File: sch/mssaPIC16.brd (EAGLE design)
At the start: 60.2 x 30 mm, 32 parts, among them IC1 PIC16F676P, IC2 7805L, Q1 BC550C, Q2 BC550C

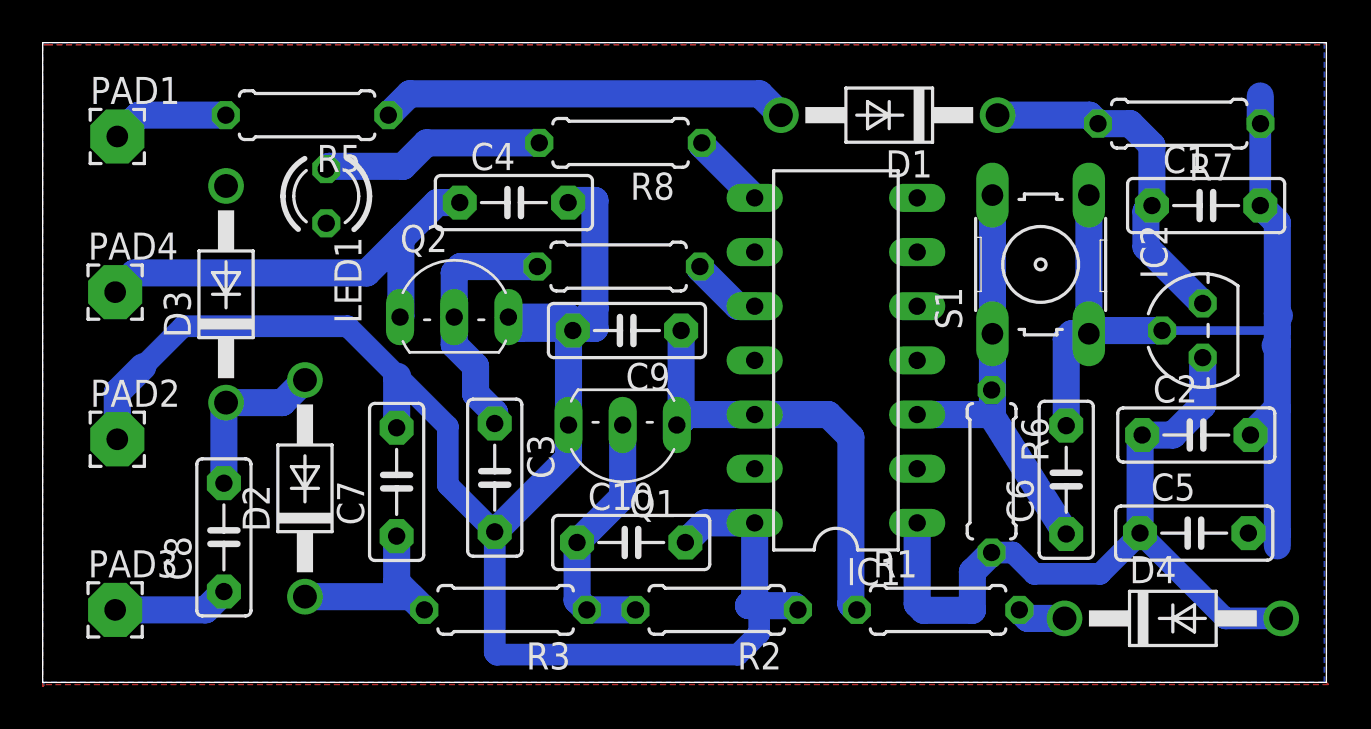
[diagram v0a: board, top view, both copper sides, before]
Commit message: SSA v.034
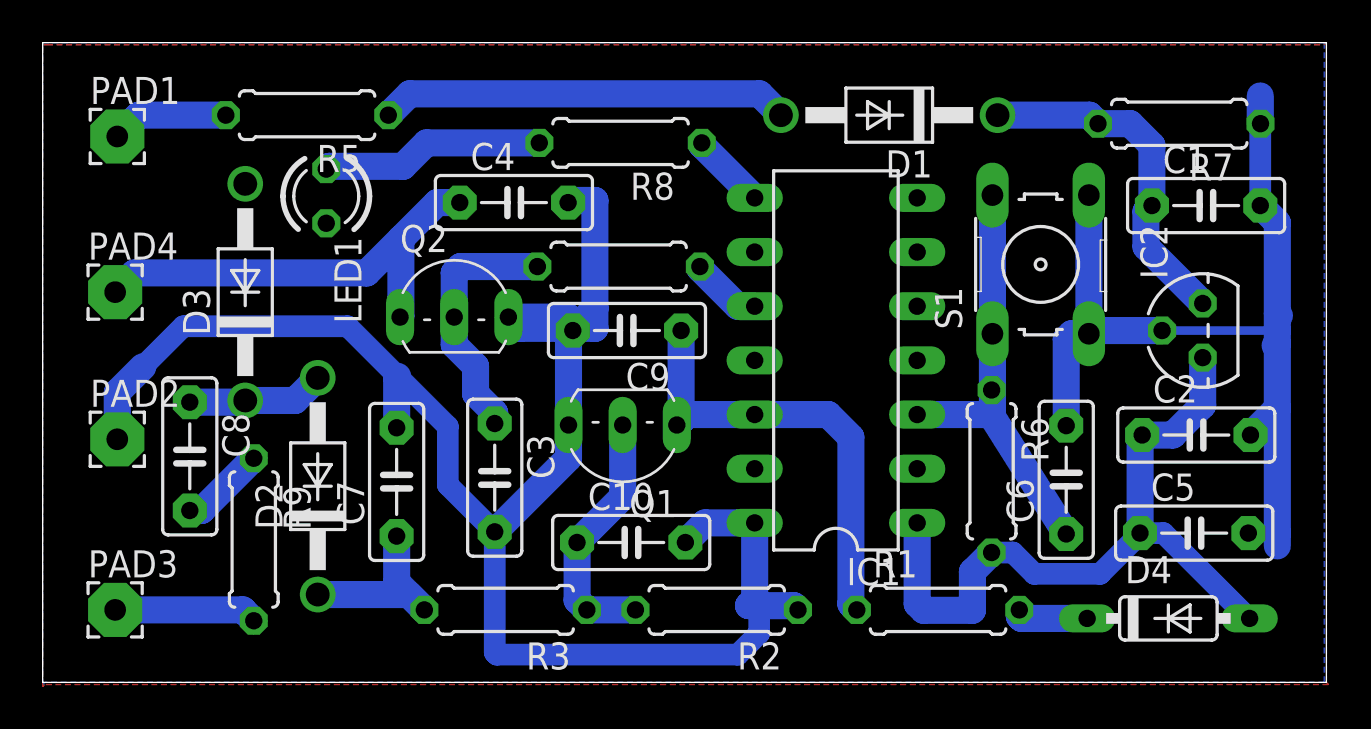
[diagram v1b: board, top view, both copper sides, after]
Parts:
- added R9: 100, rcl:0207/7
- D4: value 1N4004 -> 1N4148DO35-7; device diode:DO41-10 -> diode:DO35-7
- moved C8 4.12 mm to (6.90, 10.6), turned to 270 degrees
- moved D3 0.91 mm to (9.50, 18.3)
- moved D2 0.61 mm to (12.9, 9.20)
- moved D4 0.21 mm to (52.8, 3.00)
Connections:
- new net N$17: PAD3.1, R9.2
- net N$12: now also C8.2, R9.1; no longer C8.1, PAD3.1
- net N$13: now also C8.1; no longer C8.2
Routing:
- net N$17: track 0.00 -> 6.71 mm
- net N$2: track 36.4 -> 34.9 mm
- net N$13: track 7.96 -> 6.49 mm
- net N$12: track 5.46 -> 4.01 mm
- net N$16: track 2.29 -> 3.52 mm
- net N$9: track 9.86 -> 9.30 mm
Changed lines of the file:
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@@
 <setting verticaltext="up"/>
 </settings>
-<grid distance="1" unitdist="mm" unit="mm" style="lines" multiple="10" display="yes" altdistance="1" altunitdist="mm" altunit="mm"/>
+<grid distance="0.1" unitdist="mm" unit="mm" style="lines" multiple="10" display="yes" altdistance="1" altunitdist="mm" altunit="mm"/>
 <layers>
 <layer number="1" name="Top" color="11" fill="1" visible="yes" active="yes"/>
@@
 <attribute name="VALUE" x="19.394" y="7.368" size="1.27" layer="27" ratio="10" rot="R90"/>
 </element>
-<element name="D2" library="diode" library_urn="urn:adsk.eagle:library:210" package="DO41-10" package3d_urn="urn:adsk.eagle:package:43336/1" value="1N4004" x="12.3" y="9.1" smashed="yes" rot="R90">
-<attribute name="NAME" x="10.649" y="7.068" size="1.27" layer="25" ratio="10" rot="R90"/>
-<attribute name="POPULARITY" value="82" x="12.3" y="9.1" size="1.778" layer="27" rot="R90" display="off"/>
-<attribute name="VALUE" x="15.094" y="7.068" size="1.27" layer="27" ratio="10" rot="R90"/>
-</element>
-<element name="D3" library="diode" library_urn="urn:adsk.eagle:library:210" package="DO41-10" package3d_urn="urn:adsk.eagle:package:43336/1" value="1N4004" x="8.6" y="18.2" smashed="yes" rot="R90">
-<attribute name="NAME" x="6.949" y="16.168" size="1.27" layer="25" ratio="10" rot="R90"/>
-<attribute name="POPULARITY" value="82" x="8.6" y="18.2" size="1.778" layer="27" rot="R90" display="off"/>
-<attribute name="VALUE" x="11.394" y="16.168" size="1.27" layer="27" ratio="10" rot="R90"/>
-</element>
-<element name="C8" library="capacitor-wima" package="C5B2.5" value="220n" x="8.5" y="6.8" smashed="yes" rot="R90">
-<attribute name="NAME" x="6.976" y="4.768" size="1.27" layer="25" ratio="10" rot="R90"/>
-<attribute name="VALUE" x="11.294" y="4.768" size="1.27" layer="27" ratio="10" rot="R90"/>
+<element name="D2" library="diode" library_urn="urn:adsk.eagle:library:210" package="DO41-10" package3d_urn="urn:adsk.eagle:package:43336/1" value="1N4004" x="12.9" y="9.2" smashed="yes" rot="R90">
+<attribute name="NAME" x="11.249" y="7.168" size="1.27" layer="25" ratio="10" rot="R90"/>
+<attribute name="POPULARITY" value="82" x="12.9" y="9.2" size="1.778" layer="27" rot="R90" display="off"/>
+<attribute name="VALUE" x="15.694" y="7.168" size="1.27" layer="27" ratio="10" rot="R90"/>
+</element>
+<element name="D3" library="diode" library_urn="urn:adsk.eagle:library:210" package="DO41-10" package3d_urn="urn:adsk.eagle:package:43336/1" value="1N4004" x="9.5" y="18.3" smashed="yes" rot="R90">
+<attribute name="NAME" x="7.849" y="16.268" size="1.27" layer="25" ratio="10" rot="R90"/>
+<attribute name="POPULARITY" value="82" x="9.5" y="18.3" size="1.778" layer="27" rot="R90" display="off"/>
+<attribute name="VALUE" x="12.294" y="16.268" size="1.27" layer="27" ratio="10" rot="R90"/>
+</element>
+<element name="C8" library="capacitor-wima" package="C5B2.5" value="220n" x="6.9" y="10.6" smashed="yes" rot="R270">
+<attribute name="NAME" x="8.424" y="12.632" size="1.27" layer="25" ratio="10" rot="R270"/>
+<attribute name="VALUE" x="4.106" y="12.632" size="1.27" layer="27" ratio="10" rot="R270"/>
 </element>
 <element name="C9" library="capacitor-wima" package="C5B2.5" value="2.2u" x="27.4" y="16.5" smashed="yes" rot="R180">
@@
 <attribute name="VALUE" x="11.649" y="20.895" size="1.27" layer="27" ratio="10" rot="R270"/>
 </element>
-<element name="D4" library="diode" library_urn="urn:adsk.eagle:library:210" package="DO41-10" package3d_urn="urn:adsk.eagle:package:43336/1" value="1N4004" x="53" y="3" smashed="yes">
-<attribute name="NAME" x="50.968" y="4.651" size="1.27" layer="25" ratio="10"/>
-<attribute name="POPULARITY" value="82" x="53" y="3" size="1.778" layer="27" display="off"/>
-<attribute name="VALUE" x="50.968" y="0.206" size="1.27" layer="27" ratio="10"/>
+<element name="D4" library="diode" library_urn="urn:adsk.eagle:library:210" package="DO35-7" package3d_urn="urn:adsk.eagle:package:43339/2" value="1N4148DO35-7" x="52.79" y="3" smashed="yes">
+<attribute name="NAME" x="50.758" y="4.651" size="1.27" layer="25" ratio="10"/>
+<attribute name="POPULARITY" value="58" x="52.79" y="3" size="1.778" layer="27" display="off"/>
+<attribute name="VALUE" x="50.758" y="0.206" size="1.27" layer="27" ratio="10"/>
+</element>
+<element name="R9" library="rcl" library_urn="urn:adsk.eagle:library:334" package="0207/7" package3d_urn="urn:adsk.eagle:package:23493/2" value="100" x="9.9" y="6.7" smashed="yes" rot="R270">
+<attribute name="NAME" x="11.297" y="9.24" size="1.27" layer="25" ratio="10" rot="R270"/>
+<attribute name="POPULARITY" value="46" x="9.9" y="6.7" size="1.778" layer="27" rot="R270" display="off"/>
+<attribute name="SPICEPREFIX" value="R" x="9.9" y="6.7" size="1.778" layer="27" rot="R270" display="off"/>
+<attribute name="VALUE" x="9.3412" y="8.986" size="1.27" layer="27" ratio="10" rot="R270"/>
 </element>
 </elements>
@@
 <wire x1="44.5" y1="6.09" x2="45.5" y2="6.09" width="1.016" layer="16"/>
 <wire x1="49.59" y1="5.09" x2="51.46" y2="6.96" width="1.016" layer="16"/>
-<wire x1="58.08" y1="3" x2="55.46" y2="3" width="1.016" layer="16"/>
-<wire x1="55.46" y1="3" x2="51.46" y2="7" width="1.016" layer="16"/>
+<wire x1="56.6" y1="3" x2="56.56" y2="3" width="1.016" layer="16"/>
+<wire x1="56.56" y1="3" x2="52.56" y2="7" width="1.016" layer="16"/>
+<wire x1="52.56" y1="7" x2="51.46" y2="7" width="1.016" layer="16"/>
 </signal>
 <signal name="N$3">
@@
 <contactref element="C7" pad="1"/>
 <contactref element="D2" pad="C"/>
-<wire x1="12.3" y1="4.02" x2="17.28" y2="4.02" width="1.27" layer="16"/>
-<wire x1="17.28" y1="4.02" x2="17.9" y2="3.4" width="1.27" layer="16"/>
+<wire x1="12.9" y1="4.12" x2="17.18" y2="4.12" width="1.27" layer="16"/>
+<wire x1="17.18" y1="4.12" x2="17.9" y2="3.4" width="1.27" layer="16"/>
 <wire x1="17.9" y1="3.4" x2="16.6" y2="4.7" width="1.27" layer="16"/>
 <wire x1="16.6" y1="4.7" x2="16.6" y2="6.86" width="1.27" layer="16"/>
@@
 <contactref element="D3" pad="C"/>
 <contactref element="D2" pad="A"/>
-<contactref element="C8" pad="2"/>
-<wire x1="8.5" y1="9.34" x2="8.5" y2="13.02" width="1.27" layer="16"/>
-<wire x1="8.5" y1="13.02" x2="8.6" y2="13.12" width="1.27" layer="16"/>
-<wire x1="8.6" y1="13.12" x2="11.24" y2="13.12" width="1.27" layer="16"/>
-<wire x1="11.24" y1="13.12" x2="12.3" y2="14.18" width="1.27" layer="16"/>
-</signal>
-<signal name="N$12">
+<wire x1="9.4" y1="13.12" x2="9.5" y2="13.22" width="1.27" layer="16"/>
+<wire x1="9.5" y1="13.22" x2="11.84" y2="13.22" width="1.27" layer="16"/>
+<wire x1="11.84" y1="13.22" x2="12.9" y2="14.28" width="1.27" layer="16"/>
 <contactref element="C8" pad="1"/>
-<contactref element="PAD3" pad="1"/>
-<wire x1="3.4" y1="3.4" x2="7.64" y2="3.4" width="1.27" layer="16"/>
-<wire x1="7.64" y1="3.4" x2="8.5" y2="4.26" width="1.27" layer="16"/>
+<wire x1="6.9" y1="13.14" x2="9.38" y2="13.14" width="1.27" layer="16"/>
+<wire x1="9.38" y1="13.14" x2="9.4" y2="13.12" width="1.27" layer="16"/>
 </signal>
 <signal name="N$14">
@@
 <contactref element="R1" pad="2"/>
 <contactref element="D4" pad="C"/>
-<wire x1="45.8" y1="3.4" x2="46.2" y2="3" width="1.27" layer="16"/>
-<wire x1="46.2" y1="3" x2="47.92" y2="3" width="1.27" layer="16"/>
+<wire x1="45.8" y1="3.4" x2="45.8" y2="3.1" width="1.27" layer="16"/>
+<wire x1="45.9" y1="3" x2="45.8" y2="3.1" width="1.27" layer="16"/>
+<wire x1="45.9" y1="3" x2="48.98" y2="3" width="1.27" layer="16"/>
+</signal>
+<signal name="N$12">
+<contactref element="R9" pad="1"/>
+<contactref element="C8" pad="2"/>
+<wire x1="6.9" y1="8.06" x2="7.45" y2="8.06" width="1.27" layer="16"/>
+<wire x1="7.45" y1="8.06" x2="9.9" y2="10.51" width="1.27" layer="16"/>
+</signal>
+<signal name="N$17">
+<contactref element="R9" pad="2"/>
+<contactref element="PAD3" pad="1"/>
+<wire x1="3.4" y1="3.4" x2="9.39" y2="3.4" width="1.27" layer="16"/>
+<wire x1="9.39" y1="3.4" x2="9.9" y2="2.89" width="1.27" layer="16"/>
 </signal>
 </signals>

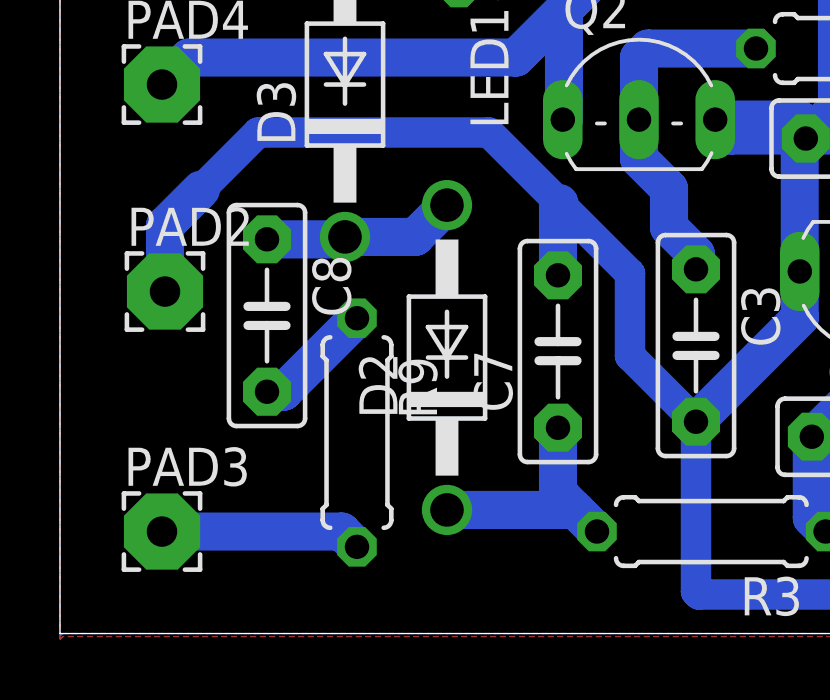
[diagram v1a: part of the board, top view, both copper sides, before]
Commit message: Add files via upload
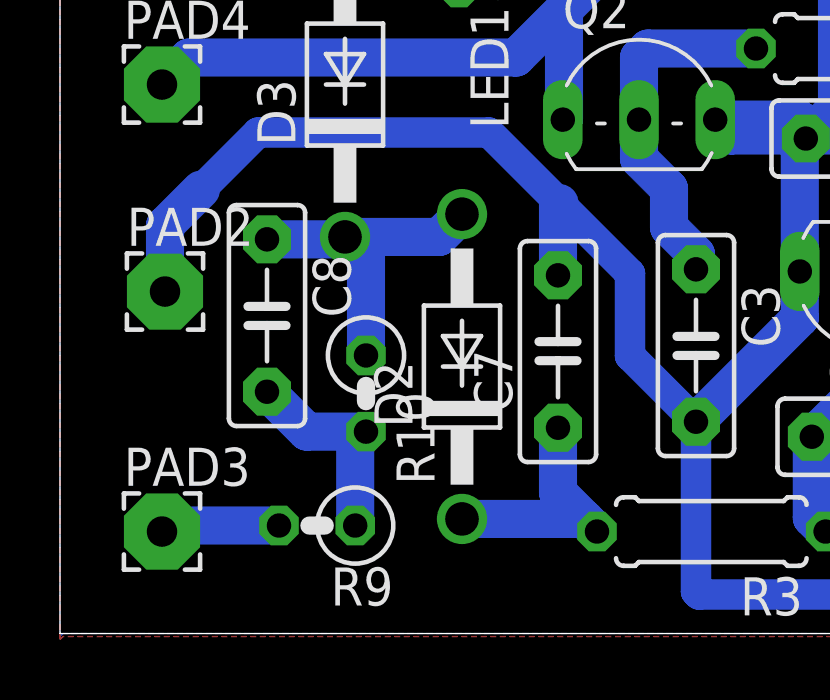
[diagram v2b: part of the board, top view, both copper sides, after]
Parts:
- added R10: 33k, rcl:0207/2V
- R1: value 15k -> 10k
- R9: device rcl:0207/7 -> rcl:0207/2V
- moved R9 3.37 mm to (8.57, 3.60), turned to 180 degrees
- moved D2 0.58 mm to (13.4, 8.90)
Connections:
- net N$12: now also R10.2
- net N$13: now also R10.1
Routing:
- net N$13: track 6.49 -> 10.9 mm
- net N$12: track 4.01 -> 7.13 mm
- net N$17: track 6.71 -> 3.98 mm
- net N$9: track 9.30 -> 8.67 mm
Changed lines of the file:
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@@
 <attribute name="VALUE" x="29.24" y="14.372" size="1.27" layer="27" ratio="10" rot="R180"/>
 </element>
-<element name="R1" library="rcl" library_urn="urn:adsk.eagle:library:334" package="0207/7" package3d_urn="urn:adsk.eagle:package:23493/2" value="15k" x="41.99" y="3.4" smashed="yes">
+<element name="R1" library="rcl" library_urn="urn:adsk.eagle:library:334" package="0207/7" package3d_urn="urn:adsk.eagle:package:23493/2" value="10k" x="41.99" y="3.4" smashed="yes">
 <attribute name="NAME" x="38.942" y="4.924" size="1.27" layer="25" ratio="10"/>
 <attribute name="POPULARITY" value="46" x="41.99" y="3.4" size="1.778" layer="27" display="off"/>
@@
 <attribute name="VALUE" x="19.394" y="7.368" size="1.27" layer="27" ratio="10" rot="R90"/>
 </element>
-<element name="D2" library="diode" library_urn="urn:adsk.eagle:library:210" package="DO41-10" package3d_urn="urn:adsk.eagle:package:43336/1" value="1N4004" x="12.9" y="9.2" smashed="yes" rot="R90">
-<attribute name="NAME" x="11.249" y="7.168" size="1.27" layer="25" ratio="10" rot="R90"/>
-<attribute name="POPULARITY" value="82" x="12.9" y="9.2" size="1.778" layer="27" rot="R90" display="off"/>
-<attribute name="VALUE" x="15.694" y="7.168" size="1.27" layer="27" ratio="10" rot="R90"/>
+<element name="D2" library="diode" library_urn="urn:adsk.eagle:library:210" package="DO41-10" package3d_urn="urn:adsk.eagle:package:43336/1" value="1N4004" x="13.4" y="8.9" smashed="yes" rot="R90">
+<attribute name="NAME" x="11.749" y="6.868" size="1.27" layer="25" ratio="10" rot="R90"/>
+<attribute name="POPULARITY" value="82" x="13.4" y="8.9" size="1.778" layer="27" rot="R90" display="off"/>
+<attribute name="VALUE" x="16.194" y="6.868" size="1.27" layer="27" ratio="10" rot="R90"/>
 </element>
 <element name="D3" library="diode" library_urn="urn:adsk.eagle:library:210" package="DO41-10" package3d_urn="urn:adsk.eagle:package:43336/1" value="1N4004" x="9.5" y="18.3" smashed="yes" rot="R90">
@@
 <attribute name="VALUE" x="50.758" y="0.206" size="1.27" layer="27" ratio="10"/>
 </element>
-<element name="R9" library="rcl" library_urn="urn:adsk.eagle:library:334" package="0207/7" package3d_urn="urn:adsk.eagle:package:23493/2" value="100" x="9.9" y="6.7" smashed="yes" rot="R270">
-<attribute name="NAME" x="11.297" y="9.24" size="1.27" layer="25" ratio="10" rot="R270"/>
-<attribute name="POPULARITY" value="46" x="9.9" y="6.7" size="1.778" layer="27" rot="R270" display="off"/>
-<attribute name="SPICEPREFIX" value="R" x="9.9" y="6.7" size="1.778" layer="27" rot="R270" display="off"/>
-<attribute name="VALUE" x="9.3412" y="8.986" size="1.27" layer="27" ratio="10" rot="R270"/>
+<element name="R9" library="rcl" library_urn="urn:adsk.eagle:library:334" package="0207/2V" package3d_urn="urn:adsk.eagle:package:23490/1" value="100" x="8.57" y="3.6" smashed="yes" rot="R180">
+<attribute name="NAME" x="11.11" y="2.203" size="1.27" layer="25" ratio="10" rot="R180"/>
+<attribute name="POPULARITY" value="17" x="8.57" y="3.6" size="1.778" layer="27" rot="R180" display="off"/>
+<attribute name="SPICEPREFIX" value="R" x="8.57" y="3.6" size="1.778" layer="27" rot="R180" display="off"/>
+<attribute name="VALUE" x="10.856" y="4.1588" size="1.27" layer="27" ratio="10" rot="R180"/>
+</element>
+<element name="R10" library="rcl" library_urn="urn:adsk.eagle:library:334" package="0207/2V" package3d_urn="urn:adsk.eagle:package:23490/1" value="33k" x="10.2" y="8" smashed="yes" rot="R270">
+<attribute name="NAME" x="11.216" y="8.0508" size="1.27" layer="25" ratio="10" rot="R270"/>
+<attribute name="POPULARITY" value="17" x="10.2" y="8" size="1.778" layer="27" rot="R270" display="off"/>
+<attribute name="SPICEPREFIX" value="R" x="10.2" y="8" size="1.778" layer="27" rot="R270" display="off"/>
+<attribute name="VALUE" x="7.9648" y="8.0508" size="1.27" layer="27" ratio="10" rot="R270"/>
 </element>
 </elements>
@@
 <contactref element="C7" pad="1"/>
 <contactref element="D2" pad="C"/>
-<wire x1="12.9" y1="4.12" x2="17.18" y2="4.12" width="1.27" layer="16"/>
-<wire x1="17.18" y1="4.12" x2="17.9" y2="3.4" width="1.27" layer="16"/>
+<wire x1="13.4" y1="3.82" x2="17.48" y2="3.82" width="1.27" layer="16"/>
+<wire x1="17.48" y1="3.82" x2="17.9" y2="3.4" width="1.27" layer="16"/>
 <wire x1="17.9" y1="3.4" x2="16.6" y2="4.7" width="1.27" layer="16"/>
 <wire x1="16.6" y1="4.7" x2="16.6" y2="6.86" width="1.27" layer="16"/>
@@
 <contactref element="D2" pad="A"/>
 <wire x1="9.4" y1="13.12" x2="9.5" y2="13.22" width="1.27" layer="16"/>
-<wire x1="9.5" y1="13.22" x2="11.84" y2="13.22" width="1.27" layer="16"/>
-<wire x1="11.84" y1="13.22" x2="12.9" y2="14.28" width="1.27" layer="16"/>
+<wire x1="9.5" y1="13.22" x2="10.3" y2="13.22" width="1.27" layer="16"/>
+<wire x1="10.3" y1="13.22" x2="12.64" y2="13.22" width="1.27" layer="16"/>
+<wire x1="12.64" y1="13.22" x2="13.4" y2="13.98" width="1.27" layer="16"/>
 <contactref element="C8" pad="1"/>
 <wire x1="6.9" y1="13.14" x2="9.38" y2="13.14" width="1.27" layer="16"/>
 <wire x1="9.38" y1="13.14" x2="9.4" y2="13.12" width="1.27" layer="16"/>
+<contactref element="R10" pad="1"/>
+<wire x1="10.2" y1="9.27" x2="10.2" y2="13.12" width="1.27" layer="16"/>
+<wire x1="10.2" y1="13.12" x2="10.3" y2="13.22" width="1.27" layer="16"/>
 </signal>
 <signal name="N$14">
@@
 <contactref element="R9" pad="1"/>
 <contactref element="C8" pad="2"/>
-<wire x1="6.9" y1="8.06" x2="7.45" y2="8.06" width="1.27" layer="16"/>
-<wire x1="7.45" y1="8.06" x2="9.9" y2="10.51" width="1.27" layer="16"/>
+<contactref element="R10" pad="2"/>
+<wire x1="10.2" y1="6.73" x2="8.23" y2="6.73" width="1.27" layer="16"/>
+<wire x1="8.23" y1="6.73" x2="6.9" y2="8.06" width="1.27" layer="16"/>
+<wire x1="9.84" y1="3.6" x2="9.84" y2="6.37" width="1.27" layer="16"/>
+<wire x1="9.84" y1="6.37" x2="10.2" y2="6.73" width="1.27" layer="16"/>
 </signal>
 <signal name="N$17">
 <contactref element="R9" pad="2"/>
 <contactref element="PAD3" pad="1"/>
-<wire x1="3.4" y1="3.4" x2="9.39" y2="3.4" width="1.27" layer="16"/>
-<wire x1="9.39" y1="3.4" x2="9.9" y2="2.89" width="1.27" layer="16"/>
+<wire x1="7.3" y1="3.6" x2="3.6" y2="3.6" width="1.27" layer="16"/>
+<wire x1="3.6" y1="3.6" x2="3.4" y2="3.4" width="1.27" layer="16"/>
 </signal>
 </signals>

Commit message: Add files via upload
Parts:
- C7: value 220n -> 470n
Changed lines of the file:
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@@
 <attribute name="VALUE" x="50.794" y="7.468" size="1.27" layer="27" ratio="10" rot="R90"/>
 </element>
-<element name="C7" library="capacitor-wima" package="C5B2.5" value="220n" x="16.6" y="9.4" smashed="yes" rot="R90">
+<element name="C7" library="capacitor-wima" package="C5B2.5" value="470n" x="16.6" y="9.4" smashed="yes" rot="R90">
 <attribute name="NAME" x="15.076" y="7.368" size="1.27" layer="25" ratio="10" rot="R90"/>
 <attribute name="VALUE" x="19.394" y="7.368" size="1.27" layer="27" ratio="10" rot="R90"/>
